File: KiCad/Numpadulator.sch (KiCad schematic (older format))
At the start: 74 parts, among them SW1 Cherry_MX_RGB_WS2812, SW10 Cherry_MX_RGB_WS2812, SW11 Cherry_MX_RGB_WS2812, SW12 Cherry_MX_RGB_WS2812, SW13 Cherry_MX_RGB_WS2812, SW14 Cherry_MX_RGB_WS2812, SW15 Cherry_MX_RGB_WS2812, SW16 Cherry_MX_RGB_WS2812, SW19 Rotary_Encoder_Switch, SW2 Cherry_MX_RGB_WS2812, SW3 Cherry_MX_RGB_WS2812, SW4 Cherry_MX_RGB_WS2812, SW5 Cherry_MX_RGB_WS2812, SW7 Cherry_MX_RGB_WS2812, SW8 Cherry_MX_RGB_WS2812, SW9 Cherry_MX_RGB_WS2812, U1 PRO_MICRO_C, U2 OLED_SSD1306

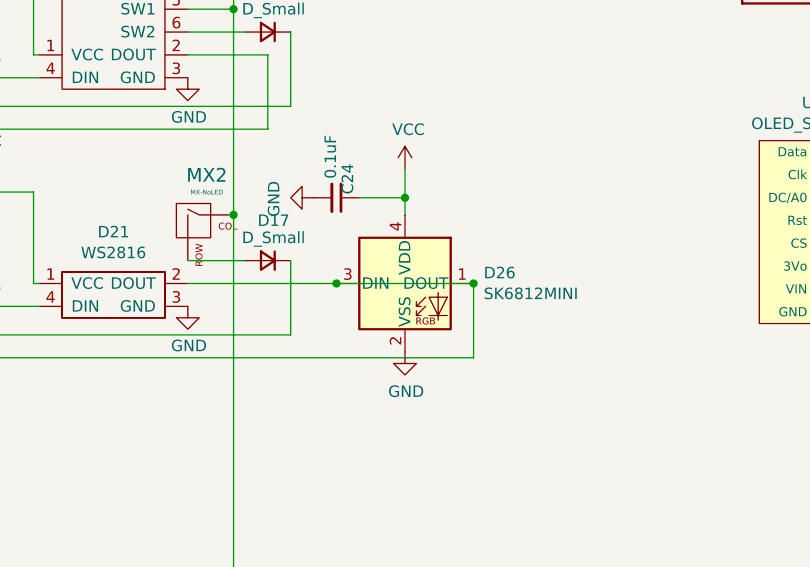
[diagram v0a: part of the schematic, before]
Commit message: PLACED EVERYTHING I THINK
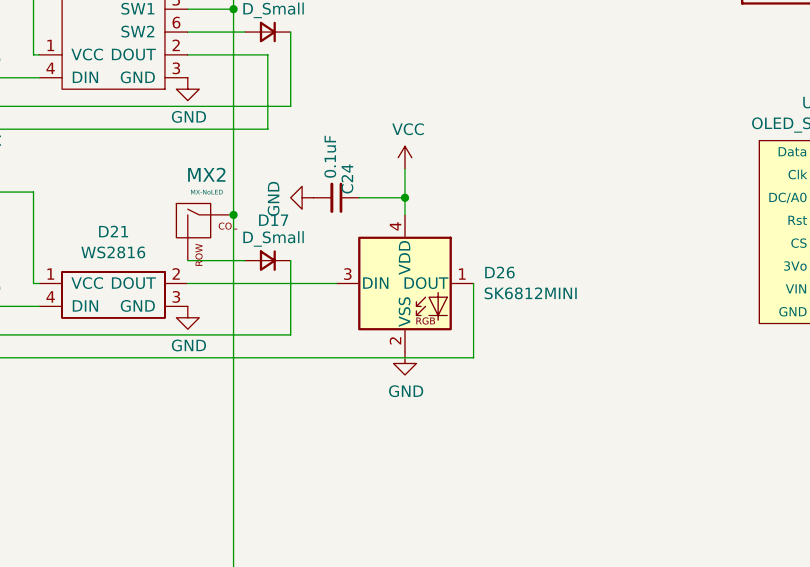
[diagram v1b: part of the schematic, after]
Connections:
- net at D21.2 (DOUT), D26.3 (DIN): no longer D26.1 (DOUT), SW4.4 (DIN)
- new net: D26.1 (DOUT), SW4.4 (DIN)
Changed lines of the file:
@@
-$EndComp
-$Comp
-L LED:SK6812MINI D26
-U 1 1 6034FC1B
-P 7825 3300
-F 0 "D26" H 8169 3346 50  0000 L CNN
-F 1 "SK6812MINI" H 8169 3255 50  0000 L CNN
-F 2 "LED_SMD:LED_SK6812MINI_PLCC4_3.5x3.5mm_P1.75mm" H 7875 3000 50  0001 L TNN
-F 3 "https://cdn-shop.adafruit.com/product-files/2686/SK6812MINI_REV.01-1-2.pdf" H 7925 2925 50  0001 L TNN
-	1    7825 3300
-	1    0    0    -1
 $EndComp
 $Comp
@@
 $EndComp
 Wire Wire Line
-	7525 3300 8125 3300
-Wire Wire Line
-	6875 3300 7525 3300
-Connection ~ 7525 3300
-Wire Wire Line
 	8125 3300 8125 3625
 Wire Wire Line
 	1075 3625 8125 3625
-Connection ~ 8125 3300
 $Comp
 L Numpadulator-rescue:C_Small-Device C24
@@
 $EndComp
 NoConn ~ 6350 6300
+Wire Wire Line
+	6875 3300 7525 3300
+$Comp
+L LED:SK6812MINI D26
+U 1 1 6034FC1B
+P 7825 3300
+F 0 "D26" H 8169 3346 50  0000 L CNN
+F 1 "SK6812MINI" H 8169 3255 50  0000 L CNN
+F 2 "LED_SMD:LED_SK6812MINI_PLCC4_3.5x3.5mm_P1.75mm" H 7875 3000 50  0001 L TNN
+F 3 "https://cdn-shop.adafruit.com/product-files/2686/SK6812MINI_REV.01-1-2.pdf" H 7925 2925 50  0001 L TNN
+	1    7825 3300
+	1    0    0    -1
+$EndComp
 $EndSCHEMATC
